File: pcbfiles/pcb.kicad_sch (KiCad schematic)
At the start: 236 parts, among them J1 Conn_01x06, J2 Conn_01x06, J3 Conn_01x06, J4 Conn_01x06, J5 Conn_01x04_Female, J6 Conn_01x04_Female, Q1 AO3401A, Q2 AO3401A, SW1 SW_SPST, SW10 SW_SPST, SW11 SW_SPST, SW12 SW_SPST, SW13 SW_SPST, SW14 SW_SPST, SW15 SW_SPST, SW16 SW_SPST, SW17 SW_SPST, SW18 SW_SPST, SW19 SW_SPST, SW2 SW_SPST, SW20 SW_SPST, SW21 SW_SPST, SW22 SW_SPST, SW23 SW_SPST, SW24 SW_SPST, SW25 SW_SPST, SW26 SW_SPST, SW27 SW_SPST, SW28 SW_SPST, SW29 SW_SPST, SW3 SW_SPST, SW30 SW_SPST, SW31 SW_SPST, SW32 SW_SPST, SW33 SW_SPST, SW34 SW_SPST, SW35 SW_SPST, SW36 SW_SPST, SW37 SW_SPST, SW38 SW_SPST, SW39 SW_SPST, SW4 SW_SPST, SW40 SW_SPST, SW41 SW_SPST, SW42 SW_SPST, SW43 SW_SPST, SW44 SW_SPST, SW45 SW_SPST, SW46 SW_SPST, SW47 SW_SPST, SW48 SW_SPST, SW49 SW_SPST, SW5 SW_SPST, SW50 SW_SPST, SW51 SW_SPST, SW52 SW_SPST, SW53 SW_SPST, SW54 SW_SPST, SW55 SW_SPST, SW56 SW_SPST, SW57 SW_SPST, SW58 SW_SPST, SW59 SW_SPST, SW6 SW_SPST, SW60 SW_SPST, SW61 SW_SPST, SW62 SW_SPST, SW63 SW_SPST, SW64 SW_SPST, SW65 SW_SPST, SW66 SW_SPST, SW67 SW_SPST, SW68 SW_SPST, SW69 SW_SPST, SW7 SW_SPST, SW70 SW_SPST, SW71 SW_SPST, SW72 SW_SPST, SW73 SW_SPST, SW74 SW_SPST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

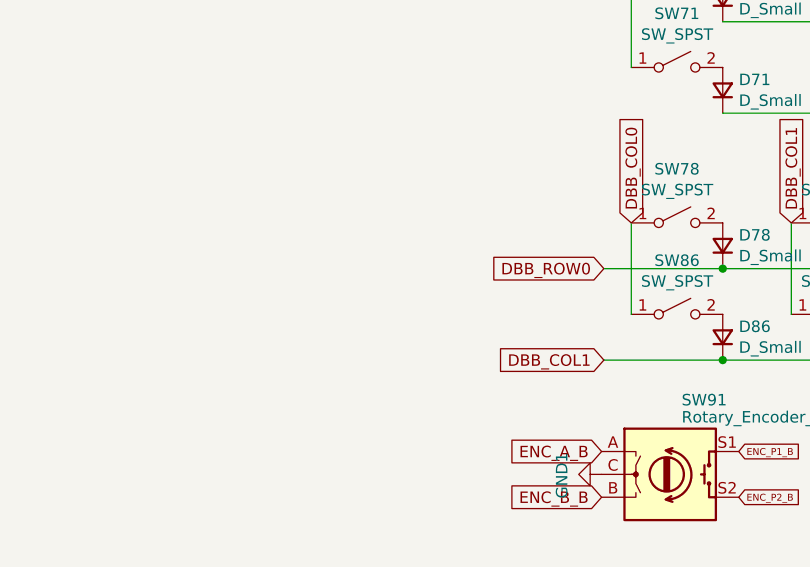
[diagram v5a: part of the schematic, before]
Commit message: Routing.
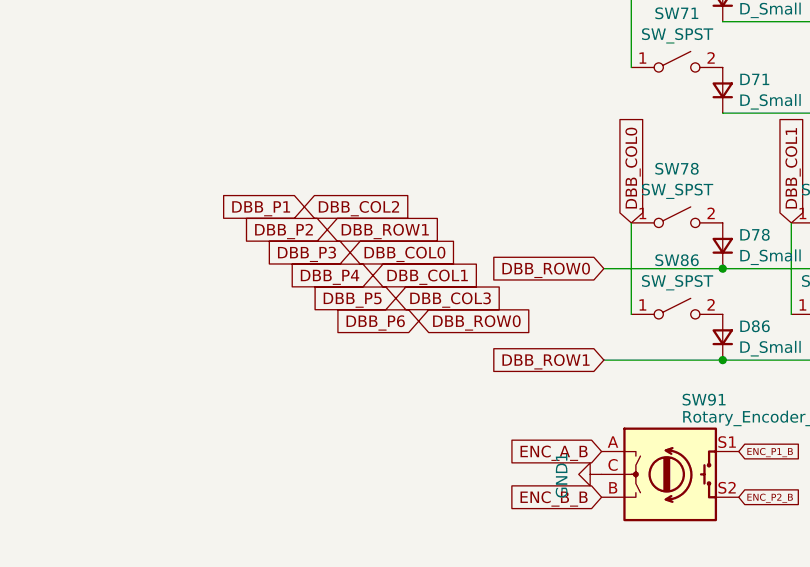
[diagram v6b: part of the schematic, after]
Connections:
- net DBB_P1 is gone; now on net DBB_COL2: J2.1 (Pin_1), J4.6 (Pin_6), U6.26 (P0.22)
- net DBB_P3 is gone; now on net DBB_COL0: J2.3 (Pin_3), J4.4 (Pin_4), U6.28 (P1.03)
- net DBB_P4 is gone; now on net DBB_COL1: J2.4 (Pin_4), J4.3 (Pin_3), U6.29 (P1.01)
- net DBB_P5 is gone; now on net DBB_COL3: J2.5 (Pin_5), J4.2 (Pin_2), U6.33 (P1.04)
- net DBB_ROW0 is gone; now on net DBB_P6: D78.1 (K), D79.1 (K), D80.1 (K), D81.1 (K)
- net DBB_COL1: no longer D86.1 (K), D87.1 (K), D88.1 (K), D89.1 (K)
- net DBB_P2: now also D86.1 (K), D87.1 (K), D88.1 (K), D89.1 (K)
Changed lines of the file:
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@@
+    )
+  )
+  (global_label "DBB_ROW1" (shape input) (at 467.36 104.648 0) (fields_autoplaced)
+    (effects (font (size 1.27 1.27)) (justify left))
+    (property "Intersheet References" "${INTERSHEET_REFS}" (id 0) (at 479.7232 104.5686 0)
+      (effects (font (size 1.27 1.27)) (justify left) hide)
     )
   )
@@
     (property "Intersheet References" "${INTERSHEET_REFS}" (id 0) (at 534.8533 273.1294 0)
       (effects (font (size 1.27 1.27)) (justify left) hide)
+    )
+  )
+  (global_label "DBB_P6" (shape input) (at 477.52 114.808 180) (fields_autoplaced)
+    (effects (font (size 1.27 1.27)) (justify right))
+    (property "Intersheet References" "${INTERSHEET_REFS}" (id 0) (at 467.9387 114.7286 0)
+      (effects (font (size 1.27 1.27)) (justify right) hide)
     )
   )
@@
     )
   )
+  (global_label "DBB_COL1" (shape input) (at 472.44 109.728 0) (fields_autoplaced)
+    (effects (font (size 1.27 1.27)) (justify left))
+    (property "Intersheet References" "${INTERSHEET_REFS}" (id 0) (at 484.3799 109.6486 0)
+      (effects (font (size 1.27 1.27)) (justify left) hide)
+    )
+  )
   (global_label "DBA_COL2" (shape input) (at 105.41 103.632 90) (fields_autoplaced)
     (effects (font (size 1.27 1.27)) (justify left))
@@
     )
   )
-  (global_label "DBB_COL1" (shape input) (at 498.094 119.126 180) (fields_autoplaced)
-    (effects (font (size 1.27 1.27)) (justify right))
-    (property "Intersheet References" "${INTERSHEET_REFS}" (id 0) (at 486.1541 119.0466 0)
+  (global_label "DBB_ROW1" (shape input) (at 498.094 119.126 180) (fields_autoplaced)
+    (effects (font (size 1.27 1.27)) (justify right))
+    (property "Intersheet References" "${INTERSHEET_REFS}" (id 0) (at 485.7308 119.0466 0)
       (effects (font (size 1.27 1.27)) (justify right) hide)
     )
@@
     )
   )
+  (global_label "DBB_P2" (shape input) (at 467.36 104.648 180) (fields_autoplaced)
+    (effects (font (size 1.27 1.27)) (justify right))
+    (property "Intersheet References" "${INTERSHEET_REFS}" (id 0) (at 457.7787 104.5686 0)
+      (effects (font (size 1.27 1.27)) (justify right) hide)
+    )
+  )
   (global_label "ENC_B_B" (shape input) (at 504.952 288.29 270) (fields_autoplaced)
     (effects (font (size 1.27 1.27)) (justify right))
@@
     )
   )
+  (global_label "DBB_ROW0" (shape input) (at 477.52 114.808 0) (fields_autoplaced)
+    (effects (font (size 1.27 1.27)) (justify left))
+    (property "Intersheet References" "${INTERSHEET_REFS}" (id 0) (at 489.8832 114.8874 0)
+      (effects (font (size 1.27 1.27)) (justify left) hide)
+    )
+  )
   (global_label "LH_COL2" (shape input) (at 69.85 25.4 90) (fields_autoplaced)
     (effects (font (size 1.27 1.27)) (justify left))
@@
     (property "Intersheet References" "${INTERSHEET_REFS}" (id 0) (at 502.4914 298.6575 90)
       (effects (font (size 1.27 1.27)) (justify right) hide)
+    )
+  )
+  (global_label "DBB_COL2" (shape input) (at 464.82 102.108 0) (fields_autoplaced)
+    (effects (font (size 1.27 1.27)) (justify left))
+    (property "Intersheet References" "${INTERSHEET_REFS}" (id 0) (at 476.7599 102.0286 0)
+      (effects (font (size 1.27 1.27)) (justify left) hide)
     )
   )
@@
     )
   )
+  (global_label "DBB_P4" (shape input) (at 472.44 109.728 180) (fields_autoplaced)
+    (effects (font (size 1.27 1.27)) (justify right))
+    (property "Intersheet References" "${INTERSHEET_REFS}" (id 0) (at 462.8587 109.6486 0)
+      (effects (font (size 1.27 1.27)) (justify right) hide)
+    )
+  )
   (global_label "DBB_COL1" (shape input) (at 518.922 103.886 90) (fields_autoplaced)
     (effects (font (size 1.27 1.27)) (justify left))
@@
     )
   )
+  (global_label "DBB_P1" (shape input) (at 464.82 102.108 180) (fields_autoplaced)
+    (effects (font (size 1.27 1.27)) (justify right))
+    (property "Intersheet References" "${INTERSHEET_REFS}" (id 0) (at 455.2387 102.0286 0)
+      (effects (font (size 1.27 1.27)) (justify right) hide)
+    )
+  )
   (global_label "LH_COL4" (shape input) (at 71.882 270.51 0) (fields_autoplaced)
     (effects (font (size 1.27 1.27)) (justify left))
@@
     )
   )
+  (global_label "DBB_P3" (shape input) (at 469.9 107.188 180) (fields_autoplaced)
+    (effects (font (size 1.27 1.27)) (justify right))
+    (property "Intersheet References" "${INTERSHEET_REFS}" (id 0) (at 460.3187 107.1086 0)
+      (effects (font (size 1.27 1.27)) (justify right) hide)
+    )
+  )
   (global_label "DBA_P5" (shape input) (at 37.846 115.316 180) (fields_autoplaced)
     (effects (font (size 1.27 1.27)) (justify right))
@@
     )
   )
+  (global_label "DBB_COL3" (shape input) (at 474.98 112.268 0) (fields_autoplaced)
+    (effects (font (size 1.27 1.27)) (justify left))
+    (property "Intersheet References" "${INTERSHEET_REFS}" (id 0) (at 486.9199 112.1886 0)
+      (effects (font (size 1.27 1.27)) (justify left) hide)
+    )
+  )
   (global_label "ENC_A" (shape input) (at 49.022 288.29 270) (fields_autoplaced)
     (effects (font (size 1.27 1.27)) (justify right))
@@
     (property "Intersheet References" "${INTERSHEET_REFS}" (id 0) (at 34.2106 14.9115 90)
       (effects (font (size 1.27 1.27)) (justify left) hide)
+    )
+  )
+  (global_label "DBB_P5" (shape input) (at 474.98 112.268 180) (fields_autoplaced)
+    (effects (font (size 1.27 1.27)) (justify right))
+    (property "Intersheet References" "${INTERSHEET_REFS}" (id 0) (at 465.3987 112.1886 0)
+      (effects (font (size 1.27 1.27)) (justify right) hide)
     )
   )
@@
     )
   )
+  (global_label "DBB_COL0" (shape input) (at 469.9 107.188 0) (fields_autoplaced)
+    (effects (font (size 1.27 1.27)) (justify left))
+    (property "Intersheet References" "${INTERSHEET_REFS}" (id 0) (at 481.8399 107.1086 0)
+      (effects (font (size 1.27 1.27)) (justify left) hide)
+    )
+  )
